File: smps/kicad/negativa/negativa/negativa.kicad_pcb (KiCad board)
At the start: 2 copper layers, 129.5 x 82.5 mm, 18 parts, among them J1 Conn_01x01_Female, J2 Conn_01x01_Female, J3 Conn_01x01_Female, J4 Conn_01x01_Female, Q1 2N3906, U1 LM2577T-ADJ

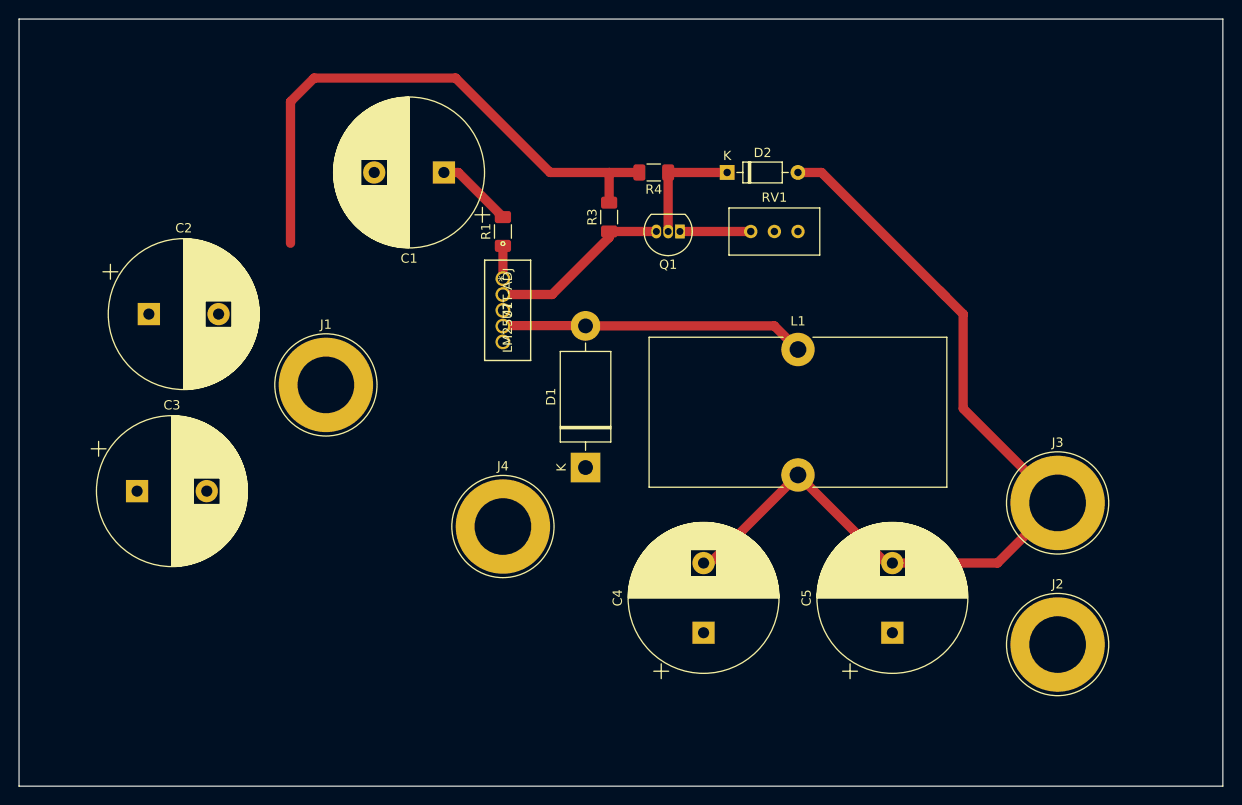
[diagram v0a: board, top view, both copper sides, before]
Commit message: varias cosas, layouts de fuentes terminados, calculo de componentes completo
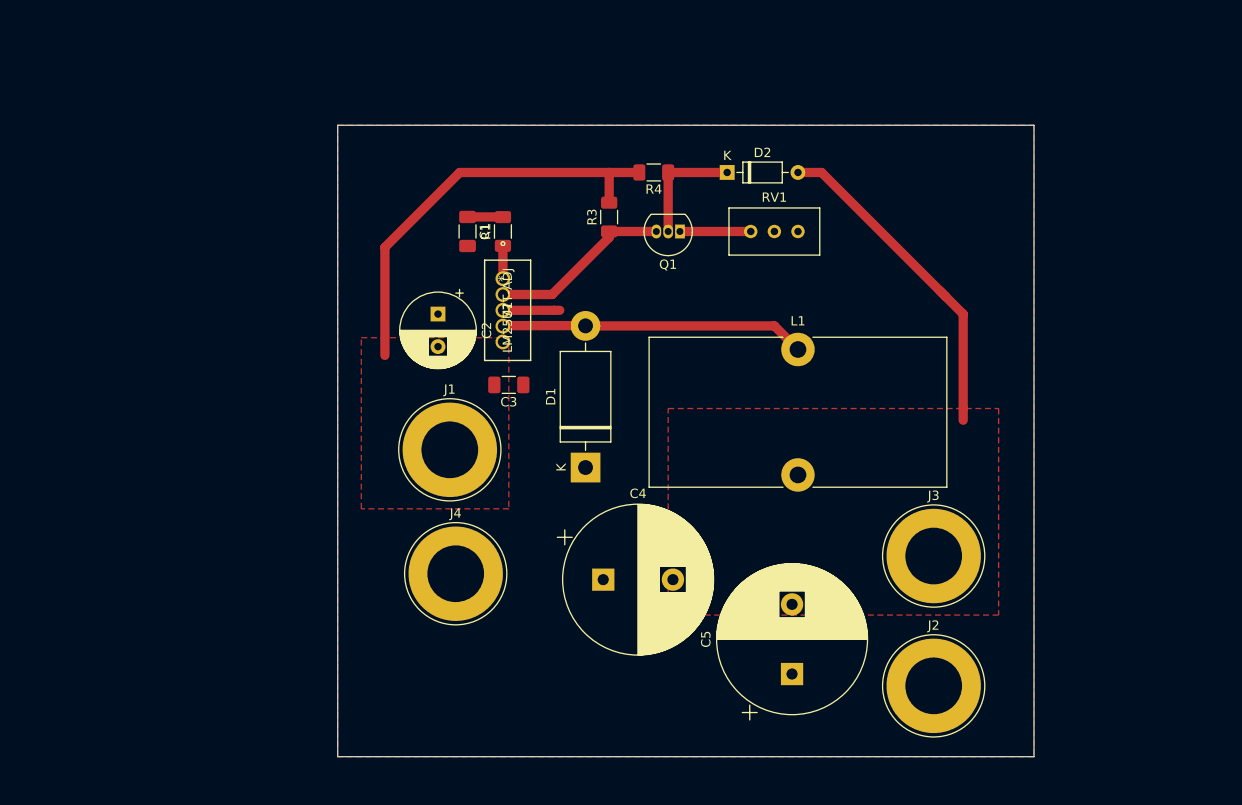
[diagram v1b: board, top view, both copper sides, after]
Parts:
- C1: footprint Capacitor_THT:CP_Radial_D16.0mm_P7.50mm -> Capacitor_SMD:C_1206_3216Metric_Pad1.33x1.80mm_HandSolder
- C2: footprint Capacitor_THT:CP_Radial_D16.0mm_P7.50mm -> Capacitor_THT:CP_Radial_D8.0mm_P3.50mm
- C3: value 100u -> 0.22u; footprint Capacitor_THT:CP_Radial_D16.0mm_P7.50mm -> Capacitor_SMD:C_1206_3216Metric_Pad1.33x1.80mm_HandSolder
- R3: value 4.12k -> 4.3k
- moved C3 41.6 mm to (136.5, 114.3), turned to 180 degrees
- moved C2 31.1 mm to (128.9, 106.7), turned to 270 degrees
- moved J1 15.1 mm to (130.2, 121.3)
- moved J3 14.5 mm to (182.2, 132.7)
- moved J2 14.1 mm to (182.2, 146.7)
- moved C4 12.2 mm to (146.7, 135.3), turned to 0 degrees
- moved C5 11.7 mm to (167.0, 145.4)
- moved J4 7.18 mm to (130.8, 134.6)
- moved C1 6.84 mm to (132.1, 97.8), turned to 270 degrees
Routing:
- net /Vout: track 102.4 -> 36.4 mm
- net /Vin: track 61.3 -> 45.6 mm
- net GND: track 0.00 -> 6.12 mm
- net Net-(C1-Pad1): track 8.34 -> 3.82 mm
- added copper zone on F.Cu, net /Vin
- added copper zone on F.Cu, net /Vout
- added copper zone on F.Cu, net GND
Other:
- board size 129.5 x 82.5 mm -> 74.9 x 67.9 mm
